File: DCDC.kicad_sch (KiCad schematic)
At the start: 25 parts, among them U5 LM76005RNPR

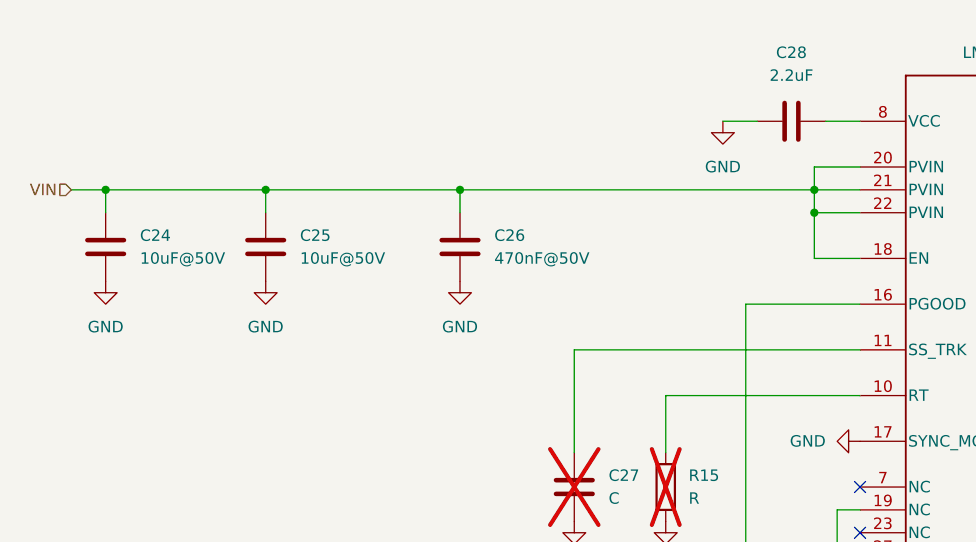
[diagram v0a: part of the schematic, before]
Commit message: Prepare v0.2
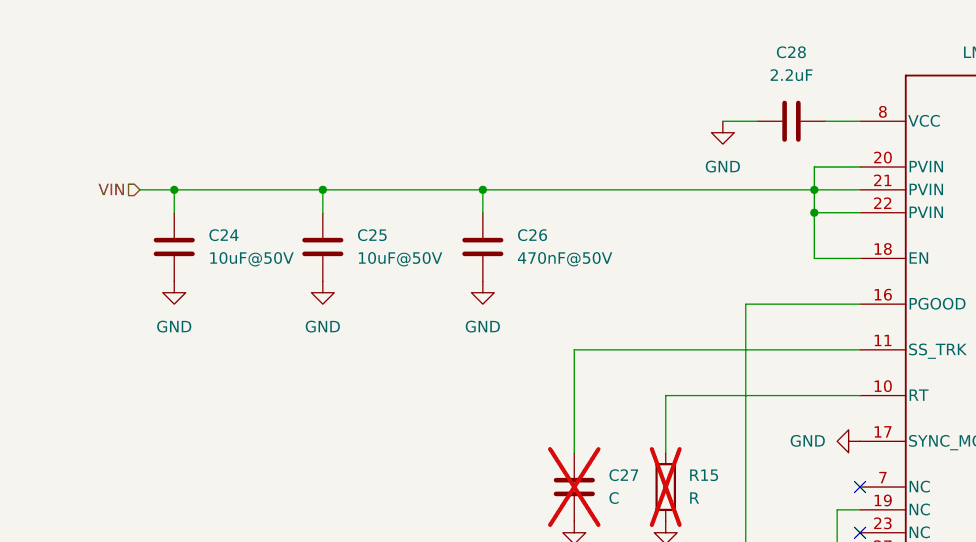
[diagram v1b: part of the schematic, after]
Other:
- moved on the sheet: C24, C25, C26
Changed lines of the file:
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@@
 	(title_block
 		(title "OpenMower SABO Mainboard for Series I & II")
-		(date "2025-02-26")
-		(rev "v0.1")
+		(date "2025-05-04")
+		(rev "v0.2")
 		(company "Apeheanger <joerg@ebeling.ws> for OpenMower")
 		(comment 1 "This design is licensed under CC BY-NC 4.0")
@@
 	)
 	(junction
-		(at 76.2 118.11)
+		(at 83.82 118.11)
 		(diameter 0)
 		(color 0 0 0 0)
@@
 	)
 	(junction
-		(at 115.57 118.11)
+		(at 118.11 118.11)
 		(diameter 0)
 		(color 0 0 0 0)
 	)
 	(junction
-		(at 93.98 118.11)
+		(at 100.33 118.11)
 		(diameter 0)
 		(color 0 0 0 0)
@@
 	(wire
 		(pts
-			(xy 115.57 118.11) (xy 154.94 118.11)
+			(xy 118.11 118.11) (xy 154.94 118.11)
 		)
 		(stroke
@@
 	(wire
 		(pts
-			(xy 93.98 118.11) (xy 115.57 118.11)
+			(xy 100.33 118.11) (xy 118.11 118.11)
 		)
 		(stroke
@@
 	(wire
 		(pts
-			(xy 93.98 118.11) (xy 93.98 120.65)
+			(xy 100.33 118.11) (xy 100.33 120.65)
 		)
 		(stroke
@@
 	(wire
 		(pts
-			(xy 76.2 118.11) (xy 76.2 120.65)
+			(xy 83.82 118.11) (xy 83.82 120.65)
 		)
 		(stroke
@@
 	(wire
 		(pts
-			(xy 72.39 118.11) (xy 76.2 118.11)
+			(xy 80.01 118.11) (xy 83.82 118.11)
 		)
 		(stroke
@@
 	(wire
 		(pts
-			(xy 115.57 118.11) (xy 115.57 120.65)
+			(xy 118.11 118.11) (xy 118.11 120.65)
 		)
 		(stroke
@@
 	(wire
 		(pts
-			(xy 76.2 118.11) (xy 93.98 118.11)
+			(xy 83.82 118.11) (xy 100.33 118.11)
 		)
 		(stroke
@@
 	(hierarchical_label "VIN"
 		(shape input)
-		(at 72.39 118.11 180)
+		(at 80.01 118.11 180)
 		(effects
 			(font
@@
 	(symbol
 		(lib_id "Device:C")
-		(at 76.2 124.46 0)
+		(at 83.82 124.46 0)
 		(unit 1)
 		(exclude_from_sim no)
@@
 		(fields_autoplaced yes)
 		(property "Reference" "C24"
-			(at 80.01 123.1899 0)
+			(at 87.63 123.1899 0)
 			(effects
 				(font
@@
 		)
 		(property "Value" "10uF@50V"
-			(at 80.01 125.7299 0)
+			(at 87.63 125.7299 0)
 			(effects
 				(font
@@
 		)
 		(property "Footprint" "Capacitor_SMD:C_1206_3216Metric"
-			(at 77.1652 128.27 0)
+			(at 84.7852 128.27 0)
 			(effects
 				(font
@@
 		)
 		(property "Datasheet" "~"
-			(at 76.2 124.46 0)
+			(at 83.82 124.46 0)
 			(effects
 				(font
@@
 		)
 		(property "Description" "Unpolarized capacitor"
-			(at 76.2 124.46 0)
+			(at 83.82 124.46 0)
 			(effects
 				(font
@@
 		)
 		(property "JLC" "C13585"
-			(at 76.2 124.46 0)
+			(at 83.82 124.46 0)
 			(effects
 				(font
@@
 	(symbol
 		(lib_id "Device:C")
-		(at 93.98 124.46 0)
+		(at 100.33 124.46 0)
 		(unit 1)
 		(exclude_from_sim no)
@@
 		(fields_autoplaced yes)
 		(property "Reference" "C25"
-			(at 97.79 123.1899 0)
+			(at 104.14 123.1899 0)
 			(effects
 				(font
@@
 		)
 		(property "Value" "10uF@50V"
-			(at 97.79 125.7299 0)
+			(at 104.14 125.7299 0)
 			(effects
 				(font
@@
 		)
 		(property "Footprint" "Capacitor_SMD:C_1206_3216Metric"
-			(at 94.9452 128.27 0)
+			(at 101.2952 128.27 0)
 			(effects
 				(font
@@
 		)
 		(property "Datasheet" "~"
-			(at 93.98 124.46 0)
+			(at 100.33 124.46 0)
 			(effects
 				(font
@@
 		)
 		(property "Description" "Unpolarized capacitor"
-			(at 93.98 124.46 0)
+			(at 100.33 124.46 0)
 			(effects
 				(font
@@
 		)
 		(property "JLC" "C13585"
-			(at 93.98 124.46 0)
+			(at 100.33 124.46 0)
 			(effects
 				(font
@@
 	(symbol
 		(lib_id "power:GND")
-		(at 76.2 128.27 0)
+		(at 83.82 128.27 0)
 		(unit 1)
 		(exclude_from_sim no)
@@
 		(fields_autoplaced yes)
 		(property "Reference" "#PWR038"
-			(at 76.2 134.62 0)
+			(at 83.82 134.62 0)
 			(effects
 				(font
@@
 		)
 		(property "Value" "GND"
-			(at 76.2 133.35 0)
+			(at 83.82 133.35 0)
 			(effects
 				(font
@@
 		)
 		(property "Footprint" ""
-			(at 76.2 128.27 0)
+			(at 83.82 128.27 0)
 			(effects
 				(font
@@
 		)
 		(property "Datasheet" ""
-			(at 76.2 128.27 0)
+			(at 83.82 128.27 0)
 			(effects
 				(font
@@
 		)
 		(property "Description" "Power symbol creates a global label with name \"GND\" , ground"
-			(at 76.2 128.27 0)
+			(at 83.82 128.27 0)
 			(effects
 				(font
@@
 	(symbol
 		(lib_id "power:GND")
-		(at 115.57 128.27 0)
+		(at 118.11 128.27 0)
 		(unit 1)
 		(exclude_from_sim no)
@@
 		(fields_autoplaced yes)
 		(property "Reference" "#PWR040"
-			(at 115.57 134.62 0)
+			(at 118.11 134.62 0)
 			(effects
 				(font
@@
 		)
 		(property "Value" "GND"
-			(at 115.57 133.35 0)
+			(at 118.11 133.35 0)
 			(effects
 				(font
@@
 		)
 		(property "Footprint" ""
-			(at 115.57 128.27 0)
+			(at 118.11 128.27 0)
 			(effects
 				(font
@@
 		)
 		(property "Datasheet" ""
-			(at 115.57 128.27 0)
+			(at 118.11 128.27 0)
 			(effects
 				(font
@@
 		)
 		(property "Description" "Power symbol creates a global label with name \"GND\" , ground"
-			(at 115.57 128.27 0)
+			(at 118.11 128.27 0)
 			(effects
 				(font
@@
 	(symbol
 		(lib_id "power:GND")
-		(at 93.98 128.27 0)
+		(at 100.33 128.27 0)
 		(unit 1)
 		(exclude_from_sim no)
@@
 		(fields_autoplaced yes)
 		(property "Reference" "#PWR039"
-			(at 93.98 134.62 0)
+			(at 100.33 134.62 0)
 			(effects
 				(font
@@
 		)
 		(property "Value" "GND"
-			(at 93.98 133.35 0)
+			(at 100.33 133.35 0)
 			(effects
 				(font
@@
 		)
 		(property "Footprint" ""
-			(at 93.98 128.27 0)
+			(at 100.33 128.27 0)
 			(effects
 				(font
@@
 		)
 		(property "Datasheet" ""
-			(at 93.98 128.27 0)
+			(at 100.33 128.27 0)
 			(effects
 				(font
@@
 		)
 		(property "Description" "Power symbol creates a global label with name \"GND\" , ground"
-			(at 93.98 128.27 0)
+			(at 100.33 128.27 0)
 			(effects
 				(font
@@
 	(symbol
 		(lib_id "Device:C")
-		(at 115.57 124.46 0)
+		(at 118.11 124.46 0)
 		(unit 1)
 		(exclude_from_sim no)
@@
 		(fields_autoplaced yes)
 		(property "Reference" "C26"
-			(at 119.38 123.1899 0)
+			(at 121.92 123.1899 0)
 			(effects
 				(font
@@
 		)
 		(property "Value" "470nF@50V"
-			(at 119.38 125.7299 0)
+			(at 121.92 125.7299 0)
 			(effects
 				(font
@@
 		)
 		(property "Footprint" "Capacitor_SMD:C_0805_2012Metric"
-			(at 116.5352 128.27 0)
+			(at 119.0752 128.27 0)
 			(effects
 				(font
@@
 		)
 		(property "Datasheet" "~"
-			(at 115.57 124.46 0)
+			(at 118.11 124.46 0)
 			(effects
 				(font
@@
 		)
 		(property "Description" "Unpolarized capacitor"
-			(at 115.57 124.46 0)
+			(at 118.11 124.46 0)
 			(effects
 				(font
@@
 		)
 		(property "JLC" "C13967"
-			(at 115.57 124.46 0)
+			(at 118.11 124.46 0)
 			(effects
 				(font
